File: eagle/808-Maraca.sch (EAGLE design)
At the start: 45 parts, among them IC1 TL071P, Q1 2N3904, Q2 2N3906, Q3 2N3906, Q4 2N3904, Q59 2N3904, Q60 2N3906

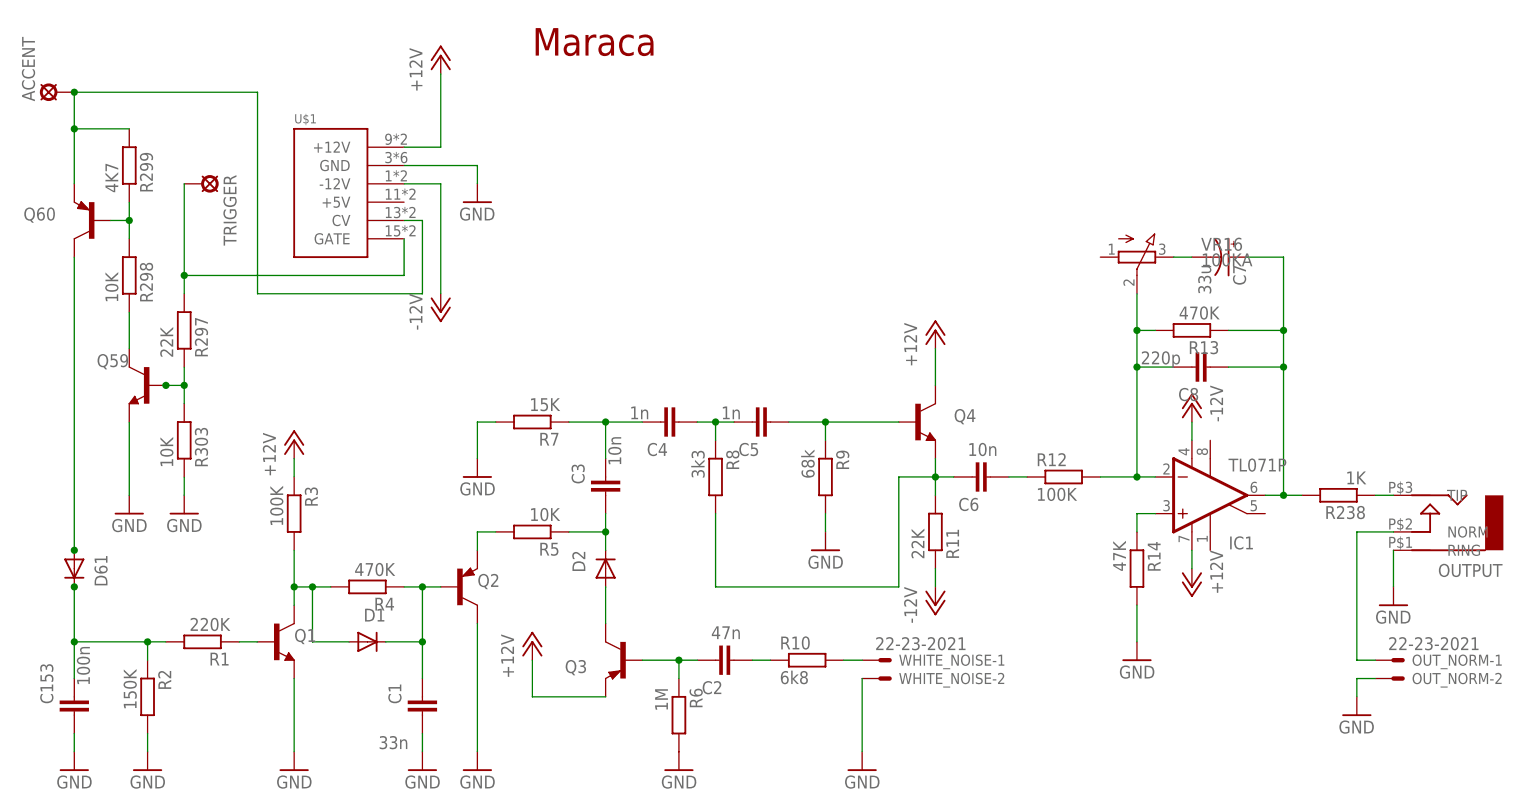
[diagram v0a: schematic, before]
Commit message: layout started
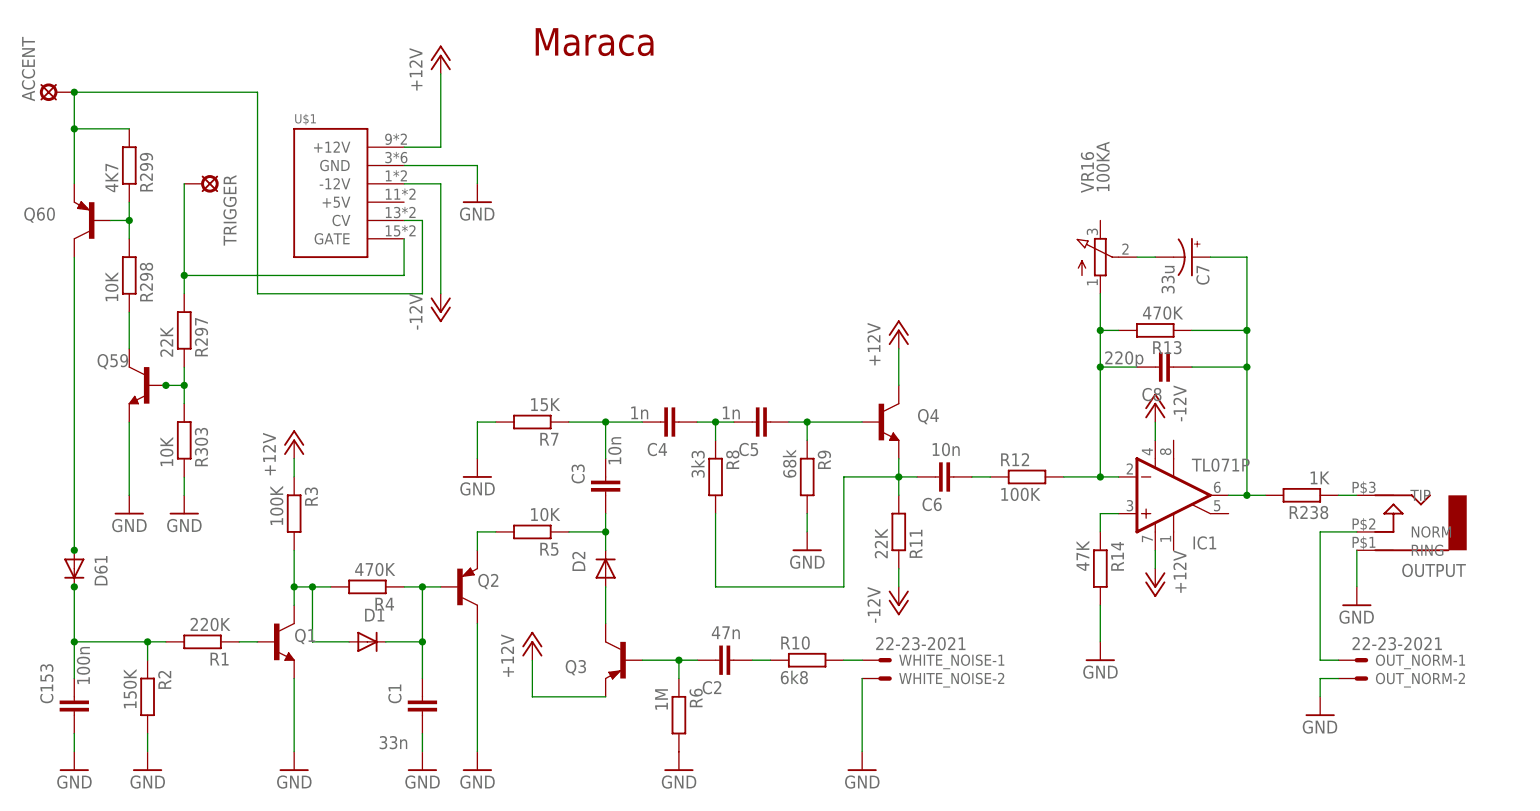
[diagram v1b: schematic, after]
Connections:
- net N$17: now also VR16.A; no longer VR16.S
- net N$19: now also VR16.S; no longer VR16.E
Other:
- moved on the sheet: C6, C7, C8, IC1, OUTPUT, OUT_NORM-1, OUT_NORM-2, Q4, R11, R12, R13, R14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

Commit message: tweaks
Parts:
- R11: device TR808clone:R-EU_0207/5V -> TR808clone:R-EU_0309/10
- R7: device TR808clone:R-EU_0207/7 -> TR808clone:R-EU_0207/5V
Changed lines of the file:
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@@
 <?xml version="1.0" encoding="utf-8"?>
 <!DOCTYPE eagle SYSTEM "eagle.dtd">
-<eagle version="7.1.0">
+<eagle version="7.2.0">
 <drawing>
 <settings>
@@
 <grid distance="0.1" unitdist="inch" unit="inch" style="lines" multiple="1" display="no" altdistance="0.01" altunitdist="inch" altunit="inch"/>
 <layers>
-<layer number="1" name="Top" color="1" fill="1" visible="no" active="no"/>
-<layer number="16" name="Bottom" color="4" fill="1" visible="no" active="no"/>
-<layer number="17" name="Pads" color="2" fill="1" visible="no" active="no"/>
-<layer number="18" name="Vias" color="2" fill="1" visible="no" active="no"/>
-<layer number="19" name="Unrouted" color="6" fill="1" visible="no" active="no"/>
-<layer number="20" name="Dimension" color="15" fill="1" visible="no" active="no"/>
-<layer number="21" name="tPlace" color="7" fill="1" visible="no" active="no"/>
-<layer number="22" name="bPlace" color="7" fill="1" visible="no" active="no"/>
-<layer number="23" name="tOrigins" color="15" fill="1" visible="no" active="no"/>
-<layer number="24" name="bOrigins" color="15" fill="1" visible="no" active="no"/>
-<layer number="25" name="tNames" color="7" fill="1" visible="no" active="no"/>
-<layer number="26" name="bNames" color="7" fill="1" visible="no" active="no"/>
-<layer number="27" name="tValues" color="7" fill="1" visible="no" active="no"/>
-<layer number="28" name="bValues" color="7" fill="1" visible="no" active="no"/>
-<layer number="29" name="tStop" color="7" fill="6" visible="no" active="no"/>
-<layer number="30" name="bStop" color="7" fill="3" visible="no" active="no"/>
-<layer number="31" name="tCream" color="7" fill="5" visible="no" active="no"/>
-<layer number="32" name="bCream" color="7" fill="4" visible="no" active="no"/>
+<layer number="1" name="Top" color="4" fill="1" visible="yes" active="no"/>
+<layer number="16" name="Bottom" color="1" fill="1" visible="yes" active="no"/>
+<layer number="17" name="Pads" color="2" fill="1" visible="yes" active="no"/>
+<layer number="18" name="Vias" color="2" fill="1" visible="yes" active="no"/>
+<layer number="19" name="Unrouted" color="6" fill="1" visible="yes" active="no"/>
+<layer number="20" name="Dimension" color="15" fill="1" visible="yes" active="no"/>
+<layer number="21" name="tPlace" color="7" fill="1" visible="yes" active="no"/>
+<layer number="22" name="bPlace" color="7" fill="1" visible="yes" active="no"/>
+<layer number="23" name="tOrigins" color="15" fill="1" visible="yes" active="no"/>
+<layer number="24" name="bOrigins" color="15" fill="1" visible="yes" active="no"/>
+<layer number="25" name="tNames" color="7" fill="1" visible="yes" active="no"/>
+<layer number="26" name="bNames" color="7" fill="1" visible="yes" active="no"/>
+<layer number="27" name="tValues" color="7" fill="1" visible="yes" active="no"/>
+<layer number="28" name="bValues" color="7" fill="1" visible="yes" active="no"/>
+<layer number="29" name="tStop" color="7" fill="3" visible="no" active="no"/>
+<layer number="30" name="bStop" color="7" fill="6" visible="no" active="no"/>
+<layer number="31" name="tCream" color="7" fill="4" visible="no" active="no"/>
+<layer number="32" name="bCream" color="7" fill="5" visible="no" active="no"/>
 <layer number="33" name="tFinish" color="6" fill="3" visible="no" active="no"/>
 <layer number="34" name="bFinish" color="6" fill="6" visible="no" active="no"/>
 <layer number="35" name="tGlue" color="7" fill="4" visible="no" active="no"/>
 <layer number="36" name="bGlue" color="7" fill="5" visible="no" active="no"/>
-<layer number="37" name="tTest" color="7" fill="1" visible="no" active="no"/>
-<layer number="38" name="bTest" color="7" fill="1" visible="no" active="no"/>
+<layer number="37" name="tTest" color="7" fill="1" visible="yes" active="no"/>
+<layer number="38" name="bTest" color="7" fill="1" visible="yes" active="no"/>
 <layer number="39" name="tKeepout" color="4" fill="11" visible="no" active="no"/>
 <layer number="40" name="bKeepout" color="1" fill="11" visible="no" active="no"/>
@@
 <layer number="44" name="Drills" color="7" fill="1" visible="no" active="no"/>
 <layer number="45" name="Holes" color="7" fill="1" visible="no" active="no"/>
-<layer number="46" name="Milling" color="3" fill="1" visible="no" active="no"/>
-<layer number="47" name="Measures" color="7" fill="1" visible="no" active="no"/>
-<layer number="48" name="Document" color="7" fill="1" visible="no" active="no"/>
-<layer number="49" name="Reference" color="7" fill="1" visible="no" active="no"/>
-<layer number="50" name="dxf" color="7" fill="1" visible="no" active="no"/>
-<layer number="51" name="tDocu" color="7" fill="1" visible="no" active="no"/>
-<layer number="52" name="bDocu" color="7" fill="1" visible="no" active="no"/>
-<layer number="53" name="tPadExt" color="7" fill="1" visible="no" active="no"/>
-<layer number="54" name="bPadExt" color="1" fill="1" visible="no" active="no"/>
-<layer number="56" name="wert" color="7" fill="1" visible="no" active="no"/>
-<layer number="57" name="tCAD" color="7" fill="1" visible="no" active="no"/>
-<layer number="59" name="tCarbon" color="7" fill="1" visible="no" active="no"/>
-<layer number="60" name="bCarbon" color="7" fill="1" visible="no" active="no"/>
+<layer number="46" name="Milling" color="3" fill="1" visible="yes" active="no"/>
+<layer number="47" name="Measures" color="7" fill="1" visible="yes" active="no"/>
+<layer number="48" name="Document" color="7" fill="1" visible="yes" active="no"/>
+<layer number="49" name="Reference" color="7" fill="1" visible="yes" active="no"/>
+<layer number="50" name="dxf" color="7" fill="1" visible="yes" active="no"/>
+<layer number="51" name="tDocu" color="7" fill="1" visible="yes" active="no"/>
+<layer number="52" name="bDocu" color="7" fill="1" visible="yes" active="no"/>
+<layer number="53" name="tPadExt" color="7" fill="1" visible="yes" active="no"/>
+<layer number="54" name="bPadExt" color="1" fill="1" visible="yes" active="no"/>
+<layer number="56" name="wert" color="7" fill="1" visible="yes" active="no"/>
+<layer number="57" name="tCAD" color="7" fill="1" visible="yes" active="no"/>
+<layer number="59" name="tCarbon" color="7" fill="1" visible="yes" active="no"/>
+<layer number="60" name="bCarbon" color="7" fill="1" visible="yes" active="no"/>
 <layer number="90" name="Modules" color="5" fill="1" visible="yes" active="yes"/>
 <layer number="91" name="Nets" color="2" fill="1" visible="yes" active="yes"/>
@@
 <part name="V9" library="supply1" deviceset="GND" device=""/>
 <part name="C3" library="TR808clone" deviceset="C-EU" device="025-025X050" value="10n"/>
-<part name="R7" library="TR808clone" deviceset="R-EU_" device="0207/7" value="15K"/>
+<part name="R7" library="TR808clone" deviceset="R-EU_" device="0207/5V" value="15K"/>
 <part name="V10" library="supply1" deviceset="GND" device=""/>
 <part name="R8" library="TR808clone" deviceset="R-EU_" device="0207/7" value="3k3"/>
@@
 <part name="V12" library="supply1" deviceset="GND" device=""/>
 <part name="Q4" library="808_lt" deviceset="2N3904" device=""/>
-<part name="R11" library="TR808clone" deviceset="R-EU_" device="0207/5V" value="22K"/>
+<part name="R11" library="TR808clone" deviceset="R-EU_" device="0309/10" value="22K"/>
 <part name="P-2" library="supply1" deviceset="-12V" device=""/>
 <part name="P+4" library="supply1" deviceset="+12V" device=""/>

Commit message: well routed
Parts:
- C5, C8: device TR808clone:C-EU025-025X050 -> TR808clone:C-EU050-024X044
- R10, R12, R238, R5, R6, R8: device TR808clone:R-EU_0207/7 -> TR808clone:R-EU_0207/5V
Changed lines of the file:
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@@
 <?xml version="1.0" encoding="utf-8"?>
 <!DOCTYPE eagle SYSTEM "eagle.dtd">
-<eagle version="7.2.0">
+<eagle version="7.1.0">
 <drawing>
 <settings>
@@
 <part name="ACCENT" library="solpad" deviceset="LSP11" device=""/>
 <part name="TRIGGER" library="solpad" deviceset="LSP11" device=""/>
-<part name="R238" library="TR808clone" deviceset="R-EU_" device="0207/7" value="1K"/>
+<part name="R238" library="TR808clone" deviceset="R-EU_" device="0207/5V" value="1K"/>
 <part name="OUTPUT" library="erthenvar" deviceset="AUDIO-JACK" device=""/>
 <part name="V4" library="supply1" deviceset="GND" device=""/>
@@
 <part name="V7" library="supply1" deviceset="GND" device=""/>
 <part name="D2" library="TR808clone" deviceset="1N4148" device="DO35-10" value="1N4148DO35-10"/>
-<part name="R5" library="TR808clone" deviceset="R-EU_" device="0207/7" value="10K"/>
+<part name="R5" library="TR808clone" deviceset="R-EU_" device="0207/5V" value="10K"/>
 <part name="V8" library="supply1" deviceset="GND" device=""/>
 <part name="Q3" library="808_lt" deviceset="2N3906" device=""/>
 <part name="P+3" library="supply1" deviceset="+12V" device=""/>
-<part name="R6" library="TR808clone" deviceset="R-EU_" device="0207/7" value="1M"/>
+<part name="R6" library="TR808clone" deviceset="R-EU_" device="0207/5V" value="1M"/>
 <part name="C2" library="TR808clone" deviceset="C-EU" device="025-025X050" value="47n"/>
 <part name="V9" library="supply1" deviceset="GND" device=""/>
@@
 <part name="R7" library="TR808clone" deviceset="R-EU_" device="0207/5V" value="15K"/>
 <part name="V10" library="supply1" deviceset="GND" device=""/>
-<part name="R8" library="TR808clone" deviceset="R-EU_" device="0207/7" value="3k3"/>
+<part name="R8" library="TR808clone" deviceset="R-EU_" device="0207/5V" value="3k3"/>
 <part name="C4" library="TR808clone" deviceset="C-EU" device="025-025X050" value="1n"/>
-<part name="C5" library="TR808clone" deviceset="C-EU" device="025-025X050" value="1n"/>
+<part name="C5" library="TR808clone" deviceset="C-EU" device="050-024X044" value="1n"/>
 <part name="V11" library="supply1" deviceset="GND" device=""/>
 <part name="R9" library="TR808clone" deviceset="R-EU_" device="0207/7" value="68k"/>
-<part name="R10" library="TR808clone" deviceset="R-EU_" device="0207/7" value="6k8"/>
+<part name="R10" library="TR808clone" deviceset="R-EU_" device="0207/5V" value="6k8"/>
 <part name="WHITE_NOISE" library="con-molex" deviceset="22-23-2021" device=""/>
 <part name="V12" library="supply1" deviceset="GND" device=""/>
@@
 <part name="P+4" library="supply1" deviceset="+12V" device=""/>
 <part name="C6" library="TR808clone" deviceset="C-EU" device="025-025X050" value="10n"/>
-<part name="R12" library="TR808clone" deviceset="R-EU_" device="0207/7" value="100K"/>
+<part name="R12" library="TR808clone" deviceset="R-EU_" device="0207/5V" value="100K"/>
 <part name="C7" library="rcl" deviceset="CPOL-US" device="B45181A" value="33u"/>
 <part name="IC1" library="linear" deviceset="TL071" device="P"/>
 <part name="R13" library="TR808clone" deviceset="R-EU_" device="0207/7" value="470K"/>
-<part name="C8" library="TR808clone" deviceset="C-EU" device="025-025X050" value="220p"/>
+<part name="C8" library="TR808clone" deviceset="C-EU" device="050-024X044" value="220p"/>
 <part name="P+5" library="supply1" deviceset="+12V" device=""/>
 <part name="P-3" library="supply1" deviceset="-12V" device=""/>
